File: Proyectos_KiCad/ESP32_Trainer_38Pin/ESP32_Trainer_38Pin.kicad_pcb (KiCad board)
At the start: 2 copper layers, 81.3 x 83.8 mm, 44 parts, among them J1 DC JACK, J2 GPIO, J3 SPI, J4 UART, J5 UART, J6 LOAD1, J7 LOAD1, Q1 2N3904, Q2 2N3904, Q3 BD139, Q4 BD139, SW1 Push, SW2 Push, U1 LM7805_TO220, U2 ESP32-38pin

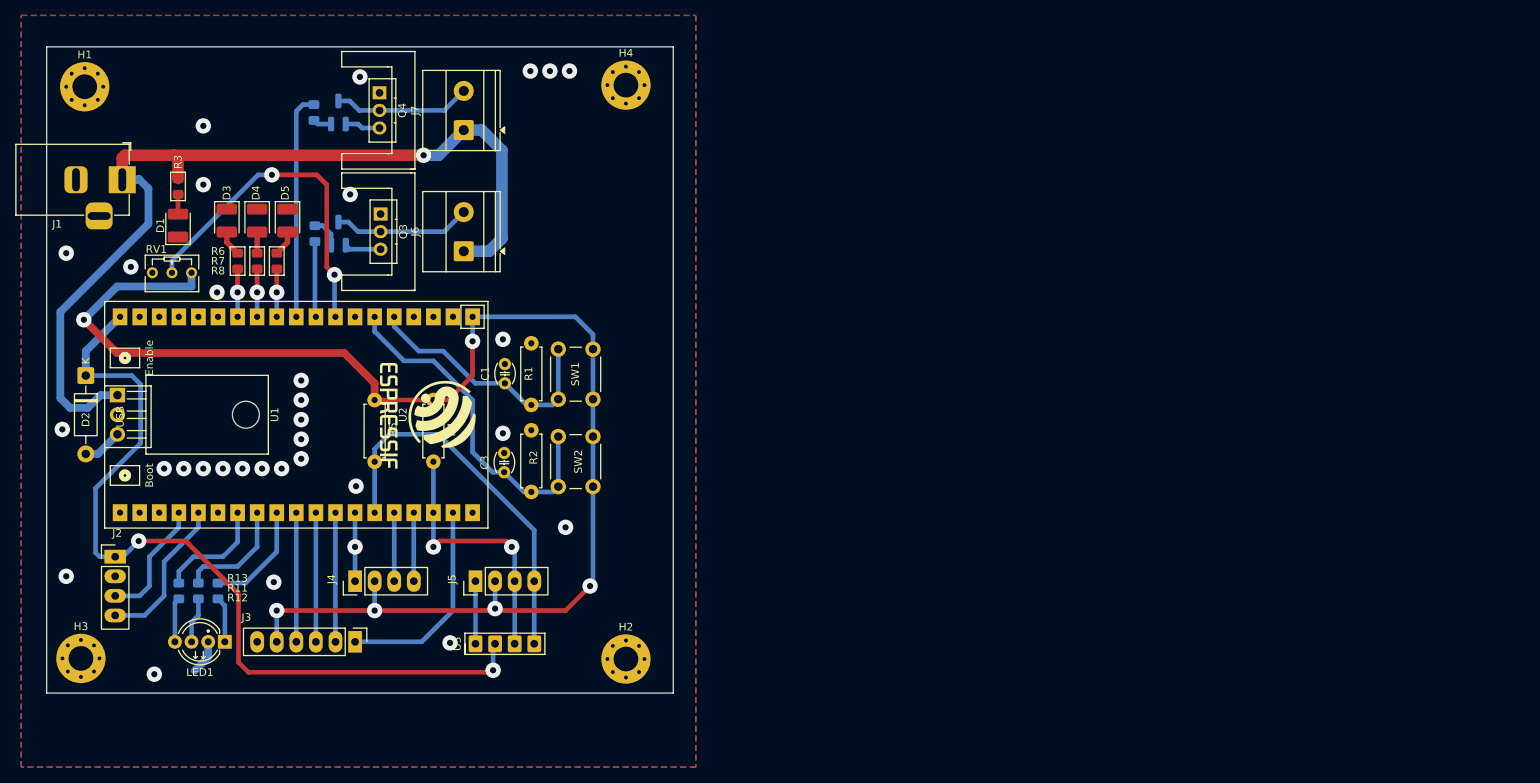
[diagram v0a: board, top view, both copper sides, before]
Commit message: Placa entrenadora esp32-38
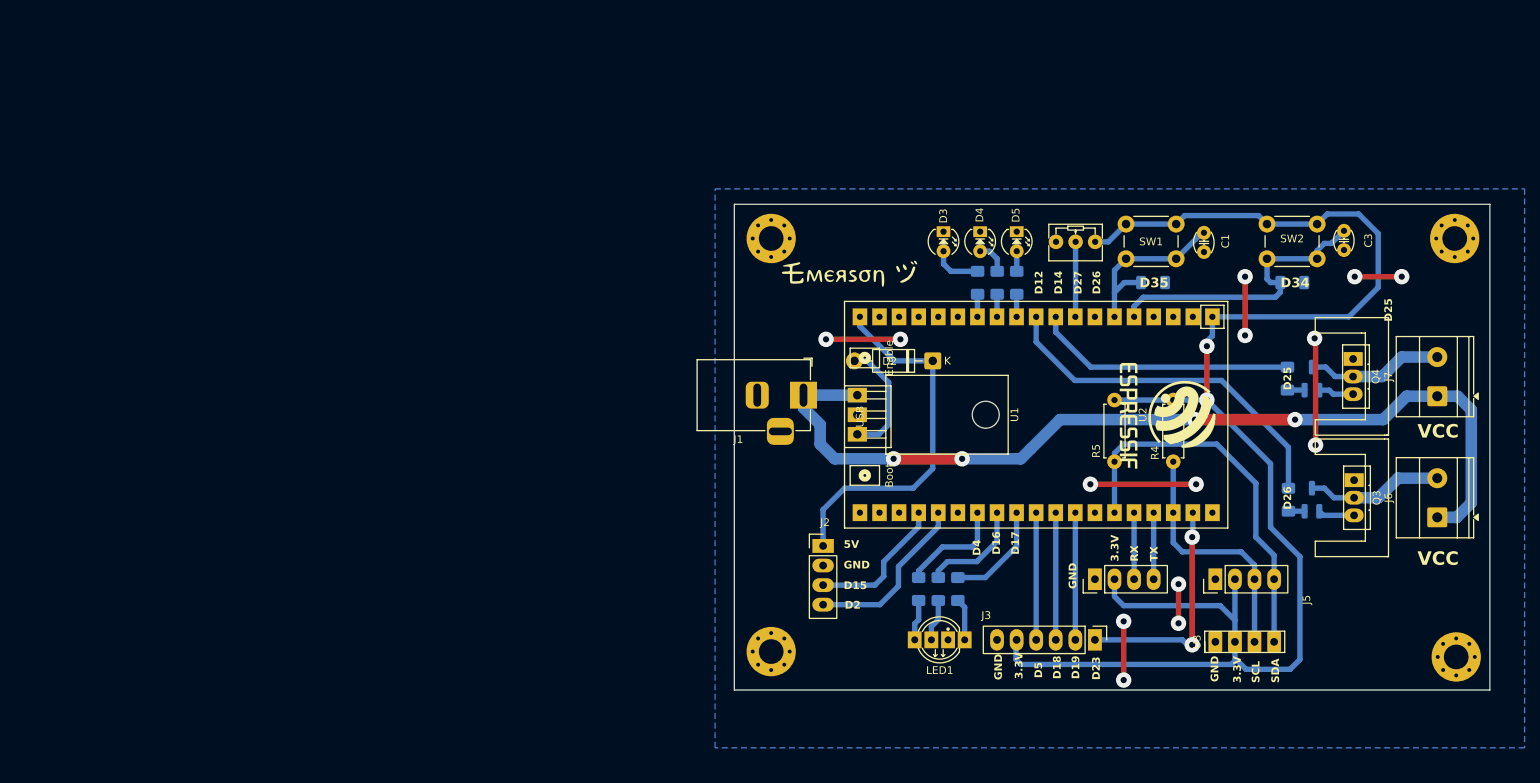
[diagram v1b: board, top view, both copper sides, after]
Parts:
- removed D1: ~, LED_SMD:LED_1210_3225Metric_Pad1.42x2.65mm_HandSolder
- removed R3: 1K, PCM_Resistor_SMD_AKL:R_0805_2012Metric_Pad1.15x1.40mm_HandSolder
- added ?: , clipboard:c932262f-0a70-4e5a-9146-f1ae92376ee6, F.Cu at (163.1, 56.3)
- D3, D4, D5: footprint LED_SMD:LED_1210_3225Metric_Pad1.42x2.65mm_HandSolder -> PCM_LED_THT_AKL:LED_D3.0mm
- R1, R2: footprint Resistencias_0.25W:470 -> PCM_Resistor_SMD_AKL:R_1206_3216Metric_Pad1.30x1.75mm_HandSolder; moved to B.Cu
- R10, R11, R12, R13, R9: footprint PCM_Resistor_SMD_AKL:R_0805_2012Metric_Pad1.15x1.40mm_HandSolder -> PCM_Resistor_SMD_AKL:R_1206_3216Metric_Pad1.42x1.75mm_HandSolder
- R6, R7, R8: footprint PCM_Resistor_SMD_AKL:R_0805_2012Metric_Pad1.15x1.40mm_HandSolder -> PCM_Resistor_SMD_AKL:R_1206_3216Metric_Pad1.42x1.75mm_HandSolder; moved to B.Cu
- moved REF** 130.9 mm to (215.3, 77.4)
- moved REF** 130.9 mm to (215.3, 61.7)
- moved J6 130.9 mm to (231.2, 87.6)
- moved J7 130.9 mm to (231.2, 71.9)
- moved Q1 130.9 mm to (214.9, 85.3)
- moved Q2 130.9 mm to (214.9, 69.6)
- moved Q3 130.9 mm to (220.4, 82.8)
- moved Q4 130.9 mm to (220.3, 67.1)
- moved R10 130.9 mm to (211.7, 69.6)
- moved R9 130.9 mm to (211.9, 85.3), turned to -90 degrees
- moved RV1 117.3 mm to (186.8, 51.9)
- moved C3 113.3 mm to (219.1, 50.4), turned to -90 degrees
- moved D2 109.9 mm to (165.7, 67.3), turned to 180 degrees
- moved H4 109.3 mm to (233.4, 51.4)
- moved H2 107.7 mm to (233.6, 105.7)
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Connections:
- C1 pad 1: PUSH_1 -> PUSH_2
- C3 pad 1: PUSH_2 -> PUSH_1
- R1 pad 1: PUSH_1 -> PUSH_2
- R10 pad 1: PWM_1 -> PWM_2
- R2 pad 1: PUSH_2 -> PUSH_1
- R9 pad 1: PWM_2 -> PWM_1
- SW1 pad 1: PUSH_1 -> PUSH_2
- SW2 pad 1: PUSH_2 -> PUSH_1
- U3 pad 2: +5V -> +3.3V
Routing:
- net +5V: track 109.8 -> 47.6 mm, vias 2 -> 0
- net GND: track 21.5 -> 63.7 mm, vias 32 -> 14
- net POT: track 44.4 -> 9.74 mm, vias 2 -> 0
- net PWM_2: track 9.82 -> 33.9 mm
- net PUSH_2: track 45.1 -> 23.6 mm
- net PWM_1: track 29.3 -> 46.9 mm
- net +3.3V: track 186.8 -> 202.6 mm, vias 6 -> 2
- net Net-(D2-A): track 5.16 -> 15.7 mm
- net PUSH_1: track 33.6 -> 39.0 mm
- net Net-(D3-A): track 3.31 -> 6.47 mm
- net MOSI: track 27.1 -> 30.1 mm, vias 0 -> 2
- net Net-(D1-A): track 2.57 -> 0.00 mm
- net GPIO2: track 20.0 -> 22.4 mm
- net GPIO15: track 16.1 -> 18.5 mm
- net LED3: track 5.32 -> 2.94 mm, vias 1 -> 0
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- removed copper zone on F.Cu, net GND
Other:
- board size 81.3 x 83.8 mm -> 98 x 63 mm
- board text added: "3.3V"
- board text added: "5V"
- board text added: "D12"
- board text added: "D14"
- board text added: "D15"
- board text added: "D16"
- board text added: "D17"
- board text added: "D18"
- board text added: "D19"
- board text added: "D2"
- board text added: "D23"
- board text added: "D25"
- board text added: "D26"
- board text added: "D27"
- board text added: "D34"
- board text added: "D35"
- board text added: "D4"
- board text added: "D5"
- board text added: "GND"
- board text added: "RX"
- board text added: "SCL"
- board text added: "SDA"
- board text added: "TX"
- board text added: "VCC"
